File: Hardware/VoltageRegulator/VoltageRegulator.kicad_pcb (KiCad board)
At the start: 2 copper layers, 22.9 x 19 mm, 9 parts, among them J1 Conn_01x04, U1 TPS7A2501DRVR

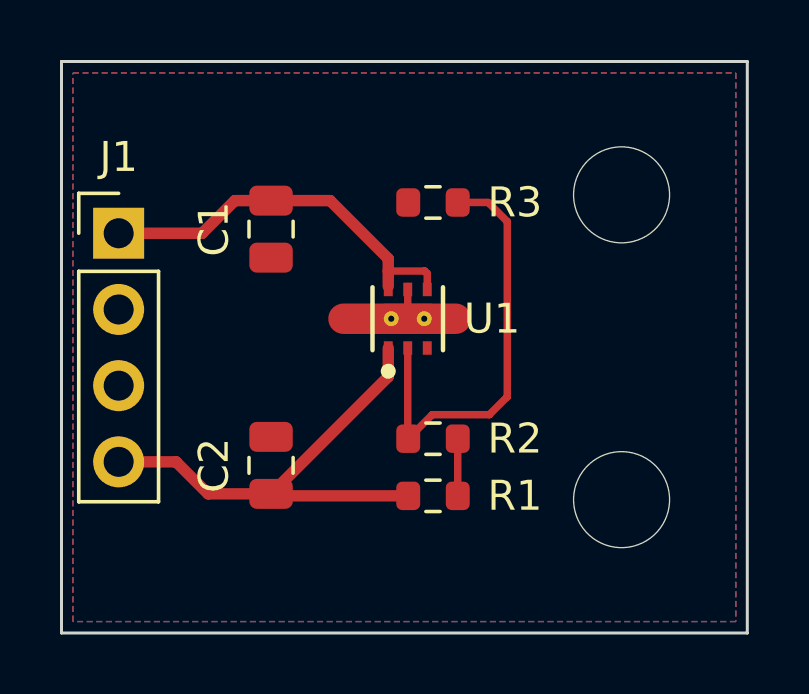
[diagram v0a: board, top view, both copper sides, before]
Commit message: Layout changes plus 3D model
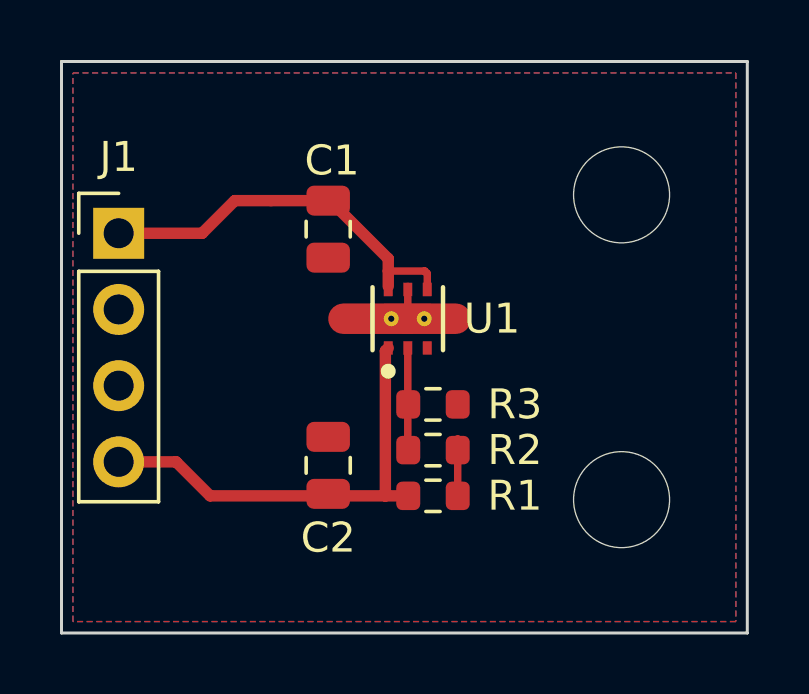
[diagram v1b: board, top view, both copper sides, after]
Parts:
- moved R3 6.73 mm to (142.6, 100.3), turned to 0 degrees
- moved C1 1.91 mm to (139.1, 94.5)
- moved C2 1.91 mm to (139.1, 102.4)
- moved R2 0.38 mm to (142.6, 101.9)
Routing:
- net Net-(U1-FB): track 14.6 -> 2.93 mm
- net VCC: track 16.6 -> 15.1 mm
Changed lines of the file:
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@@
   (net 5 "Net-(U1-FB)")
   (footprint "Capacitor_SMD:C_0805_2012Metric" (layer "F.Cu")
-    (at 137.16 94.488 -90)
+    (at 139.065 94.488 -90)
     (descr "Capacitor SMD 0805 (2012 Metric), square (rectangular) end terminal, IPC_7351 nominal, (Body size source: IPC-SM-782 page 76, https://www.pcb-3d.com/wordpress/wp-content/uploads/ipc-sm-782a_amendment_1_and_2.pdf, https://docs.google.com/spreadsheets/d/1BsfQQcO9C6DZCsRaXUlFlo91Tg2WpOkGARC1WS5S8t0/edit?usp=sharing), generated with kicad-footprint-generator")
     (tags "capacitor")
@@
     (property "ki_keywords" "cap capacitor")
     (attr smd)
-    (fp_text reference "C1" (at 0 1.905 90) (layer "F.SilkS")
-        (effects (font (size 1 1) (thickness 0.15)))
-    )
-    (fp_text value "1u" (at -2.225 1.905 90) (layer "F.Fab")
+    (fp_text reference "C1" (at -2.286 -0.127 -180) (layer "F.SilkS")
+        (effects (font (size 1 1) (thickness 0.15)))
+    )
+    (fp_text value "1u" (at -3.683 0 -180) (layer "F.Fab")
         (effects (font (size 1 1) (thickness 0.15)))
     )
@@
   )
   (footprint "Resistor_SMD:R_0603_1608Metric" (layer "F.Cu")
-    (at 142.558 101.473 180)
+    (at 142.558 101.854 180)
     (descr "Resistor SMD 0603 (1608 Metric), square (rectangular) end terminal, IPC_7351 nominal, (Body size source: IPC-SM-782 page 72, https://www.pcb-3d.com/wordpress/wp-content/uploads/ipc-sm-782a_amendment_1_and_2.pdf), generated with kicad-footprint-generator")
     (tags "resistor")
@@
   )
   (footprint "Capacitor_SMD:C_0805_2012Metric" (layer "F.Cu")
-    (at 137.16 102.362 90)
+    (at 139.065 102.362 90)
     (descr "Capacitor SMD 0805 (2012 Metric), square (rectangular) end terminal, IPC_7351 nominal, (Body size source: IPC-SM-782 page 76, https://www.pcb-3d.com/wordpress/wp-content/uploads/ipc-sm-782a_amendment_1_and_2.pdf, https://docs.google.com/spreadsheets/d/1BsfQQcO9C6DZCsRaXUlFlo91Tg2WpOkGARC1WS5S8t0/edit?usp=sharing), generated with kicad-footprint-generator")
     (tags "capacitor")
@@
     (property "ki_keywords" "cap capacitor")
     (attr smd)
-    (fp_text reference "C2" (at 0 -1.905 90) (layer "F.SilkS")
-        (effects (font (size 1 1) (thickness 0.15)))
-    )
-    (fp_text value "2.2u" (at -2.86 -1.905 90) (layer "F.Fab")
+    (fp_text reference "C2" (at -2.413 0 180) (layer "F.SilkS")
+        (effects (font (size 1 1) (thickness 0.15)))
+    )
+    (fp_text value "2.2u" (at -3.683 0 180) (layer "F.Fab")
         (effects (font (size 1 1) (thickness 0.15)))
     )
@@
   )
   (footprint "Resistor_SMD:R_0603_1608Metric" (layer "F.Cu")
-    (at 142.557 93.599 180)
+    (at 142.557 100.33)
     (descr "Resistor SMD 0603 (1608 Metric), square (rectangular) end terminal, IPC_7351 nominal, (Body size source: IPC-SM-782 page 72, https://www.pcb-3d.com/wordpress/wp-content/uploads/ipc-sm-782a_amendment_1_and_2.pdf), generated with kicad-footprint-generator")
     (tags "resistor")
@@
     (property "ki_keywords" "R res resistor")
     (attr smd)
-    (fp_text reference "R3" (at -2.731 0) (layer "F.SilkS")
-        (effects (font (size 1 1) (thickness 0.15)))
-    )
-    (fp_text value "1M" (at -5.017 0) (layer "F.Fab")
+    (fp_text reference "R3" (at 2.731 0) (layer "F.SilkS")
+        (effects (font (size 1 1) (thickness 0.15)))
+    )
+    (fp_text value "1M" (at 4.763 0) (layer "F.Fab")
         (effects (font (size 1 1) (thickness 0.15)))
     )
@@
     (fp_line (start 0.8 0.4125) (end -0.8 0.4125)
       (stroke (width 0.1) (type solid)) (layer "F.Fab"))
-    (pad "1" smd roundrect (at -0.825 0 180) (size 0.8 0.95) (layers "F.Cu" "F.Paste" "F.Mask") (roundrect_rratio 0.25)
+    (pad "1" smd roundrect (at -0.825 0) (size 0.8 0.95) (layers "F.Cu" "F.Paste" "F.Mask") (roundrect_rratio 0.25)
       (net 5 "Net-(U1-FB)") (pintype "passive"))
-    (pad "2" smd roundrect (at 0.825 0 180) (size 0.8 0.95) (layers "F.Cu" "F.Paste" "F.Mask") (roundrect_rratio 0.25)
+    (pad "2" smd roundrect (at 0.825 0) (size 0.8 0.95) (layers "F.Cu" "F.Paste" "F.Mask") (roundrect_rratio 0.25)
       (net 2 "GND") (pintype "passive"))
     (model "${KICAD6_3DMODEL_DIR}/Resistor_SMD.3dshapes/R_0603_1608Metric.wrl"
@@
     (pad "9" thru_hole circle (at 0 -0.549999 90) (size 0.499999 0.499999) (drill 0.2032) (layers "*.Cu" "*.Mask")
       (net 2 "GND") (zone_connect 2))
+    (model "${KIPRJMOD}/Libraries/TPS7A2501DRVR.pretty/DRV0006A.stp"
+      (offset (xyz 0 0 0))
+      (scale (xyz 1 1 1))
+      (rotate (xyz 0 0 0))
+    )
   )
   (footprint "MountingHole:MountingHole_3.2mm_M3" (layer "F.Cu")
@@
   (segment (start 141.716999 97.473968) (end 143.318032 97.473968) (width 1.016) (layer "F.Cu") (net 2))
   (segment (start 141.716999 96.395936) (end 141.716999 97.473968) (width 0.25) (layer "F.Cu") (net 2))
-  (segment (start 135.062 103.312) (end 137.16 103.312) (width 0.381) (layer "F.Cu") (net 3))
-  (segment (start 141.066998 98.452) (end 141.066998 99.405002) (width 0.381) (layer "F.Cu") (net 3))
-  (segment (start 137.226 103.378) (end 137.16 103.312) (width 0.381) (layer "F.Cu") (net 3))
-  (segment (start 133.995 102.245) (end 135.062 103.312) (width 0.381) (layer "F.Cu") (net 3))
-  (segment (start 141.066998 99.405002) (end 137.16 103.312) (width 0.381) (layer "F.Cu") (net 3))
+  (segment (start 140.97 98.545965) (end 140.97 103.378) (width 0.381) (layer "F.Cu") (net 3))
   (segment (start 132.08 102.245) (end 133.995 102.245) (width 0.381) (layer "F.Cu") (net 3))
-  (segment (start 141.733 103.378) (end 137.226 103.378) (width 0.381) (layer "F.Cu") (net 3))
+  (segment (start 141.066998 98.448967) (end 140.97 98.545965) (width 0.381) (layer "F.Cu") (net 3))
+  (segment (start 133.995 102.245) (end 135.128 103.378) (width 0.381) (layer "F.Cu") (net 3))
+  (segment (start 135.128 103.378) (end 140.97 103.378) (width 0.381) (layer "F.Cu") (net 3))
+  (segment (start 140.97 103.378) (end 141.733 103.378) (width 0.381) (layer "F.Cu") (net 3))
   (segment (start 143.383 103.378) (end 143.383 101.473) (width 0.25) (layer "F.Cu") (net 4))
-  (segment (start 144.437 100.673) (end 142.533 100.673) (width 0.25) (layer "F.Cu") (net 5))
   (segment (start 141.733 101.473) (end 141.716999 101.456999) (width 0.25) (layer "F.Cu") (net 5))
-  (segment (start 143.382 93.599) (end 144.399 93.599) (width 0.25) (layer "F.Cu") (net 5))
-  (segment (start 142.533 100.673) (end 141.733 101.473) (width 0.25) (layer "F.Cu") (net 5))
   (segment (start 141.716999 101.456999) (end 141.716999 98.552) (width 0.25) (layer "F.Cu") (net 5))
-  (segment (start 145.034 100.076) (end 144.437 100.673) (width 0.25) (layer "F.Cu") (net 5))
-  (segment (start 144.399 93.599) (end 145.034 94.234) (width 0.25) (layer "F.Cu") (net 5))
-  (segment (start 145.034 94.234) (end 145.034 100.076) (width 0.25) (layer "F.Cu") (net 5))
   (zone (net 2) (net_name "GND") (layer "F.Cu") (hatch edge 0.5)
     (connect_pads (clearance 0.5))
